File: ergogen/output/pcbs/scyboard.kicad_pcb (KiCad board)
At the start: 2 copper layers, 143.9 x 96.5 mm, 76 parts

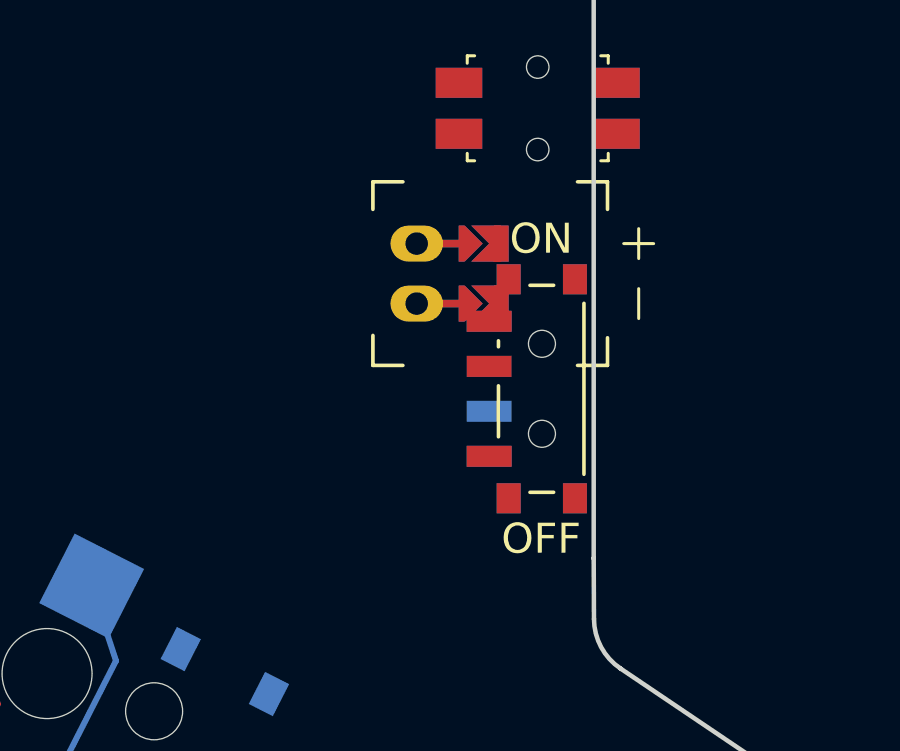
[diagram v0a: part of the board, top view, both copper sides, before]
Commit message: Compile
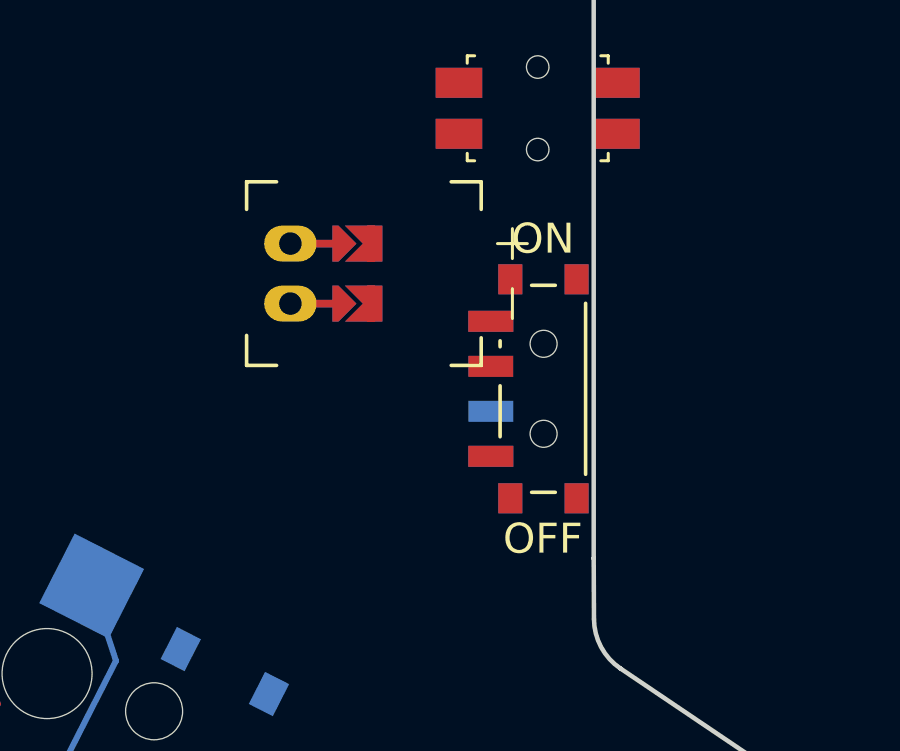
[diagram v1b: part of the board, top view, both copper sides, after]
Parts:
- moved JST1 4.21 mm to (159.6, 89.0)
- moved PWR1 0.06 mm to (168.1, 92.9)
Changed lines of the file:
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@@
   (footprint "ceoloide:power_switch_smd_side"
     (layer "F.Cu")
-    (at 168 92.87 0)
+    (at 168.055 92.87 0)
     (property "Reference" "PWR1"
       (at -3.6 0 -90)
@@
     (footprint "ceoloide:battery_connector_jst_ph_2"
         (layer "F.Cu")
-        (at 163.85 89.03 90)
+        (at 159.64 89.03 90)
         (property "Reference" "JST1"
             (at 0 4.8 90)
@@
         )
     )
-    (segment (start 165.65 90.03) (end 163.85 90.03) (width 0.25) (layer "F.Cu") (net 75))
-    (segment (start 165.65 90.03) (end 163.85 90.03) (width 0.25) (layer "B.Cu") (net 75))
-    (segment (start 165.65 88.03) (end 163.85 88.03) (width 0.25) (layer "F.Cu") (net 76))
-    (segment (start 165.65 88.03) (end 163.85 88.03) (width 0.25) (layer "B.Cu") (net 76))
+    (segment (start 161.44 90.03) (end 159.64 90.03) (width 0.25) (layer "F.Cu") (net 75))
+    (segment (start 161.44 90.03) (end 159.64 90.03) (width 0.25) (layer "B.Cu") (net 75))
+    (segment (start 161.44 88.03) (end 159.64 88.03) (width 0.25) (layer "F.Cu") (net 76))
+    (segment (start 161.44 88.03) (end 159.64 88.03) (width 0.25) (layer "B.Cu") (net 76))
   (footprint "ceoloide:mounting_hole_npth"
     (layer "F.Cu")

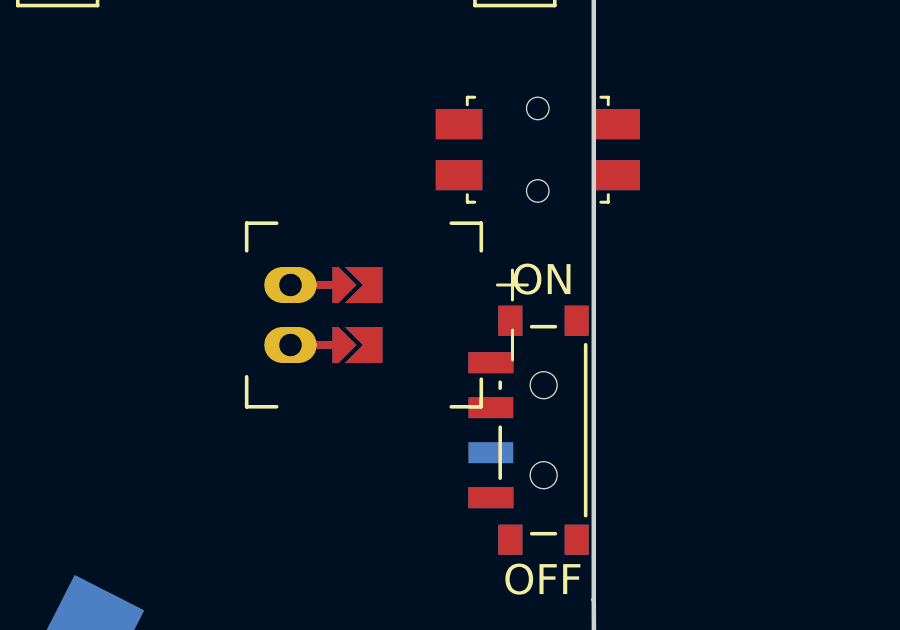
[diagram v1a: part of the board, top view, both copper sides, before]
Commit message: Compile
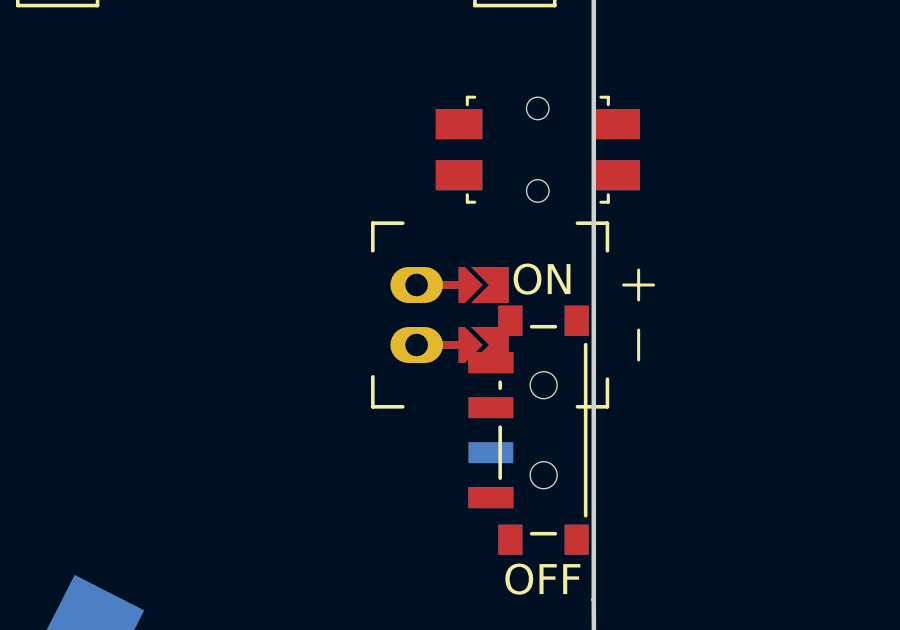
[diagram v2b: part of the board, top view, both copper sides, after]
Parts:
- moved JST1 4.21 mm to (163.8, 89.0)
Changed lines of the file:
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@@
     (footprint "ceoloide:battery_connector_jst_ph_2"
         (layer "F.Cu")
-        (at 159.64 89.03 90)
+        (at 163.845 89.03 90)
         (property "Reference" "JST1"
             (at 0 4.8 90)
@@
         )
     )
-    (segment (start 161.44 90.03) (end 159.64 90.03) (width 0.25) (layer "F.Cu") (net 75))
-    (segment (start 161.44 90.03) (end 159.64 90.03) (width 0.25) (layer "B.Cu") (net 75))
-    (segment (start 161.44 88.03) (end 159.64 88.03) (width 0.25) (layer "F.Cu") (net 76))
-    (segment (start 161.44 88.03) (end 159.64 88.03) (width 0.25) (layer "B.Cu") (net 76))
+    (segment (start 165.645 90.03) (end 163.845 90.03) (width 0.25) (layer "F.Cu") (net 75))
+    (segment (start 165.645 90.03) (end 163.845 90.03) (width 0.25) (layer "B.Cu") (net 75))
+    (segment (start 165.645 88.03) (end 163.845 88.03) (width 0.25) (layer "F.Cu") (net 76))
+    (segment (start 165.645 88.03) (end 163.845 88.03) (width 0.25) (layer "B.Cu") (net 76))
   (footprint "ceoloide:mounting_hole_npth"
     (layer "F.Cu")
